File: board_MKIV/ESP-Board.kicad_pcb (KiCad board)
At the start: 2 copper layers, 100 x 34 mm, 18 parts, among them J7 20-pin-straight, U1 ESP32-DEVKITC-32D, U6 SH-7070TB

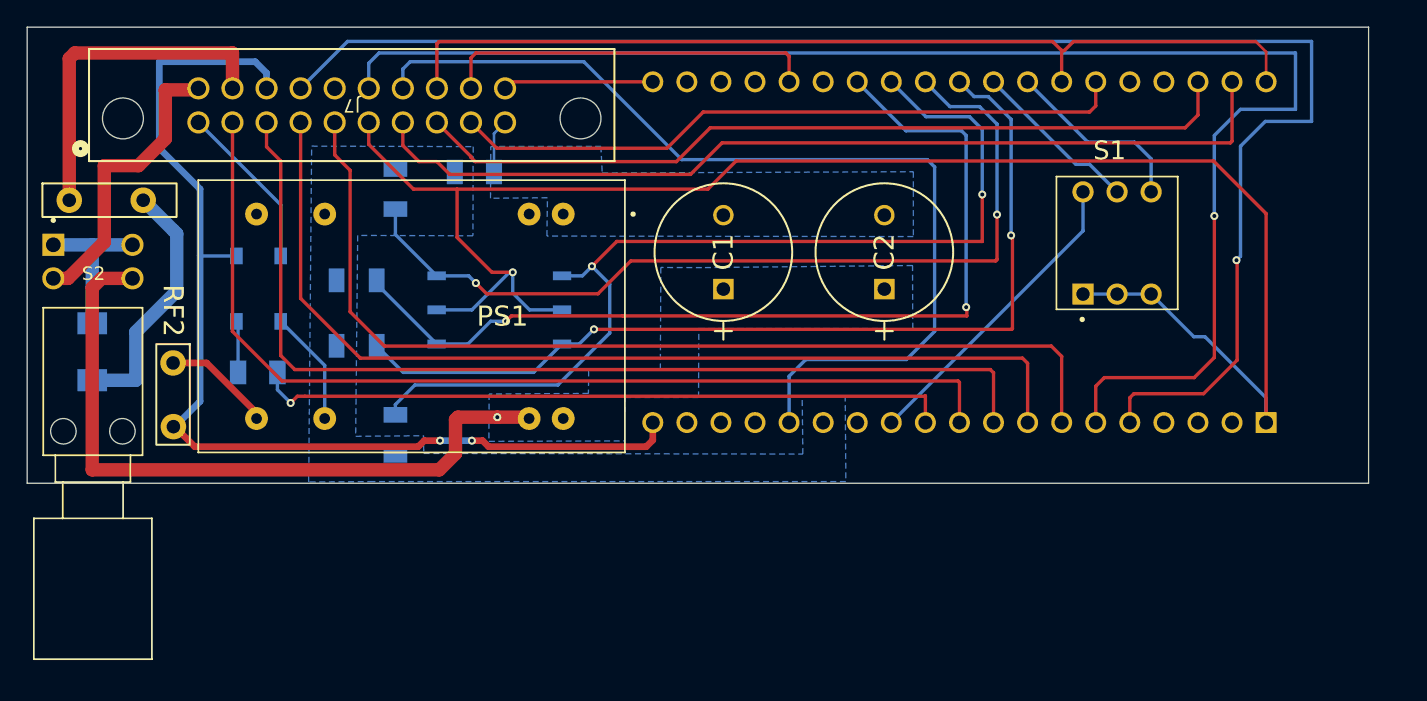
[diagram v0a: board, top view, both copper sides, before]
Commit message: MKIV Update
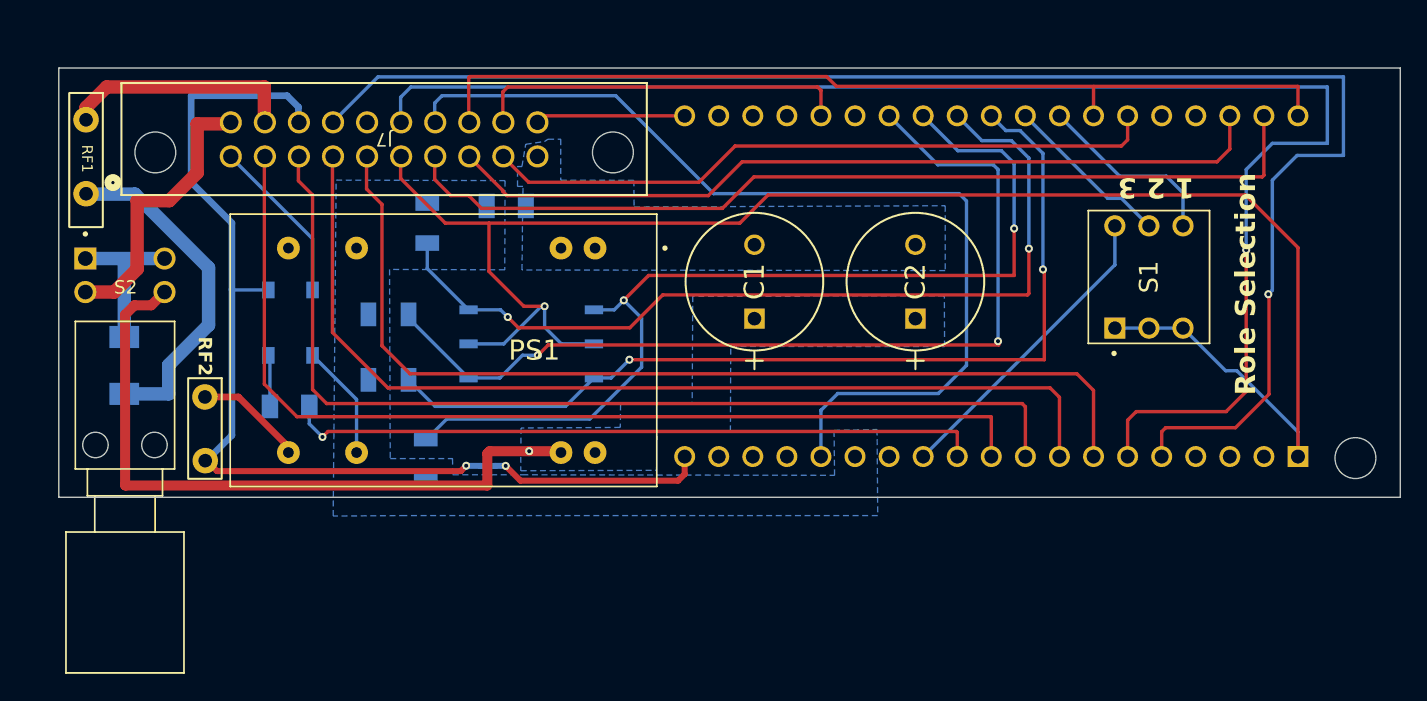
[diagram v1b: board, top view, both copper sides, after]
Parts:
- added ?: , , F.Cu at (192.9, 101.8)
- moved RF1 6.12 mm to (98.2, 76.5), turned to -90 degrees
- moved J7 3.50 mm to (109.0, 79.3)
- moved R14 3.47 mm to (120.8, 95.9)
- moved RF2 3.47 mm to (107.1, 96.8)
- moved LED1 3.47 mm to (113.5, 91.7)
- moved PS1 3.47 mm to (124.9, 93.7)
- moved R13 3.47 mm to (123.7, 84.2)
- moved R16 3.47 mm to (120.8, 91.0)
- moved R7 3.47 mm to (113.4, 97.9)
- moved S1 3.47 mm to (177.5, 88.2)
- moved U1 3.47 mm to (168.8, 88.9)
- moved U6 3.47 mm to (131.4, 93.2)
- moved C3 3.47 mm to (129.6, 83.0)
- moved C1 3.20 mm to (148.1, 91.4)
- moved C2 3.20 mm to (160.1, 91.4)
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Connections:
- net /+VOUT renamed /ESP-Board/+VOUT
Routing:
- net +VIN-dc: track 25.3 -> 17.5 mm
- net +VIN: track 94.0 -> 98.1 mm
- net -Vin: track 4.03 -> 0.00 mm
- net GPIO_26: track 74.3 -> 75.1 mm
- net ESP_GND2: track 79.2 -> 78.5 mm
- net GPIO_16: track 74.0 -> 73.4 mm
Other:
- board size 100 x 34 mm -> 100 x 32 mm
- board text added: "1 2 3"
- board text added: "ID"
- board text added: "Role Selection"
